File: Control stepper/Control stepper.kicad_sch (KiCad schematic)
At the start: 12 parts, among them J1 Conn_01x04, J2 Conn_01x02, J3 Conn_01x03, Q1 2n2222a, Q2 2n2222a, Q3 2n2222a, Q4 2n2222a, U1 4017

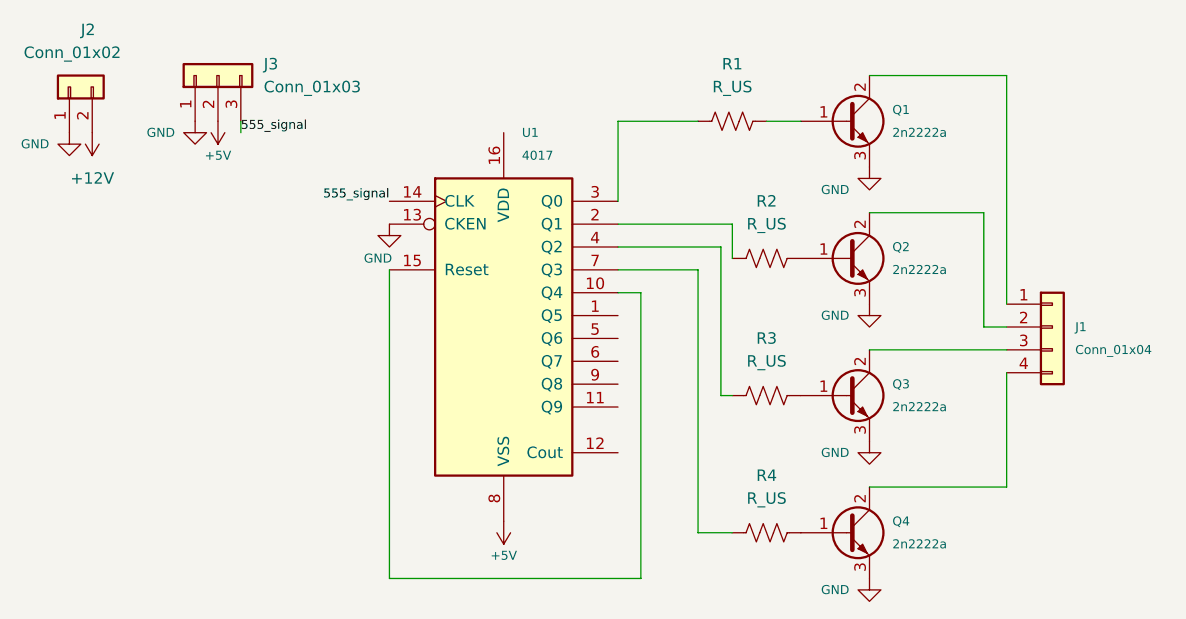
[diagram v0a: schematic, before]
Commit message: final
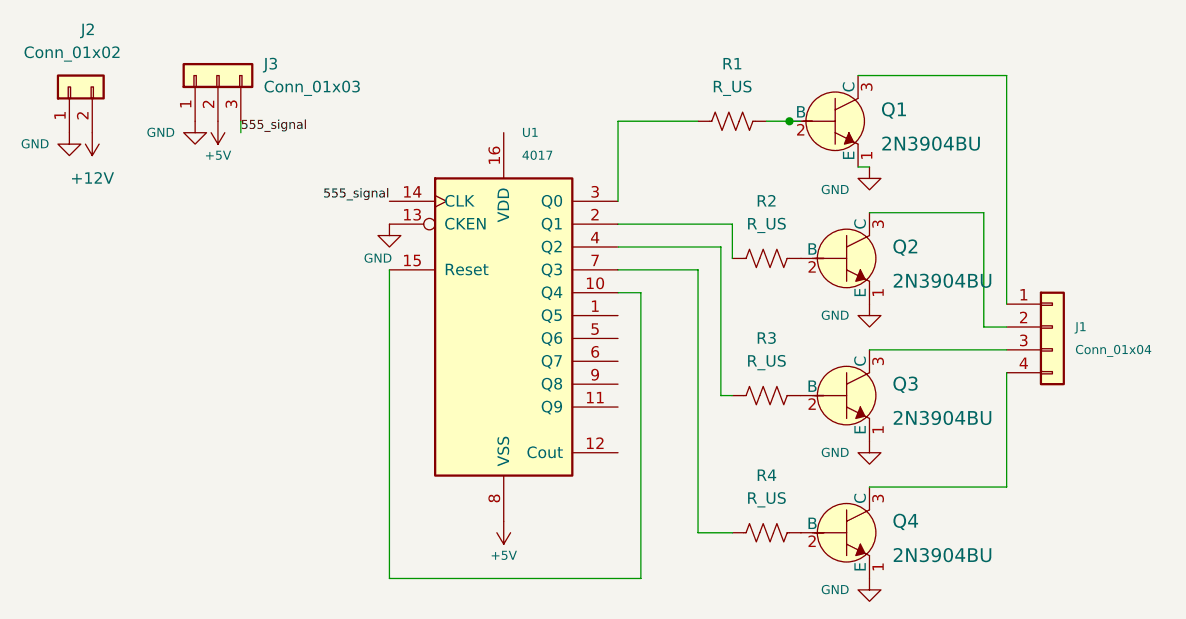
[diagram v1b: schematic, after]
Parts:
- removed Q1, Q2, Q3, Q4: 2n2222a, Package_TO_SOT_THT:TO-92, symbol Transistor_BJT:2SD1047
- added Q1, Q2, Q3, Q4: 2N3904BU, Package_TO_SOT_THT:TO-92, symbol dk_Transistors-Bipolar-BJT-Single:2N3904BU
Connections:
- net GND: now also Q1.1 (E), Q2.1 (E), Q3.1 (E), Q4.1 (E)
- net at R1.1: now also Q1.2 (B)
- net at R3.1: now also Q3.2 (B)
- net at J1.3 (Pin_3): now also Q3.3 (C)
- net at R4.1: now also Q4.2 (B)
- net at J1.4 (Pin_4): now also Q4.3 (C)
- net at R2.1: now also Q2.2 (B)
- net at J1.2 (Pin_2): now also Q2.3 (C)
- net at J1.1 (Pin_1): now also Q1.3 (C)
